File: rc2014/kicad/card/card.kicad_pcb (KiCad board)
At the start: 4 copper layers, 63.5 x 102.6 mm, 27 parts, among them J1 Conn_RC40_Male, J2 DB15_Female_HighDensity, J3 Conn_02x06_Top_Bottom, SW1 SW_DIP_x07, U1 74HCT688, U2 SN74LVC8T245PWR, U3 SN74LVC8T245PWR, U4 VDC-II

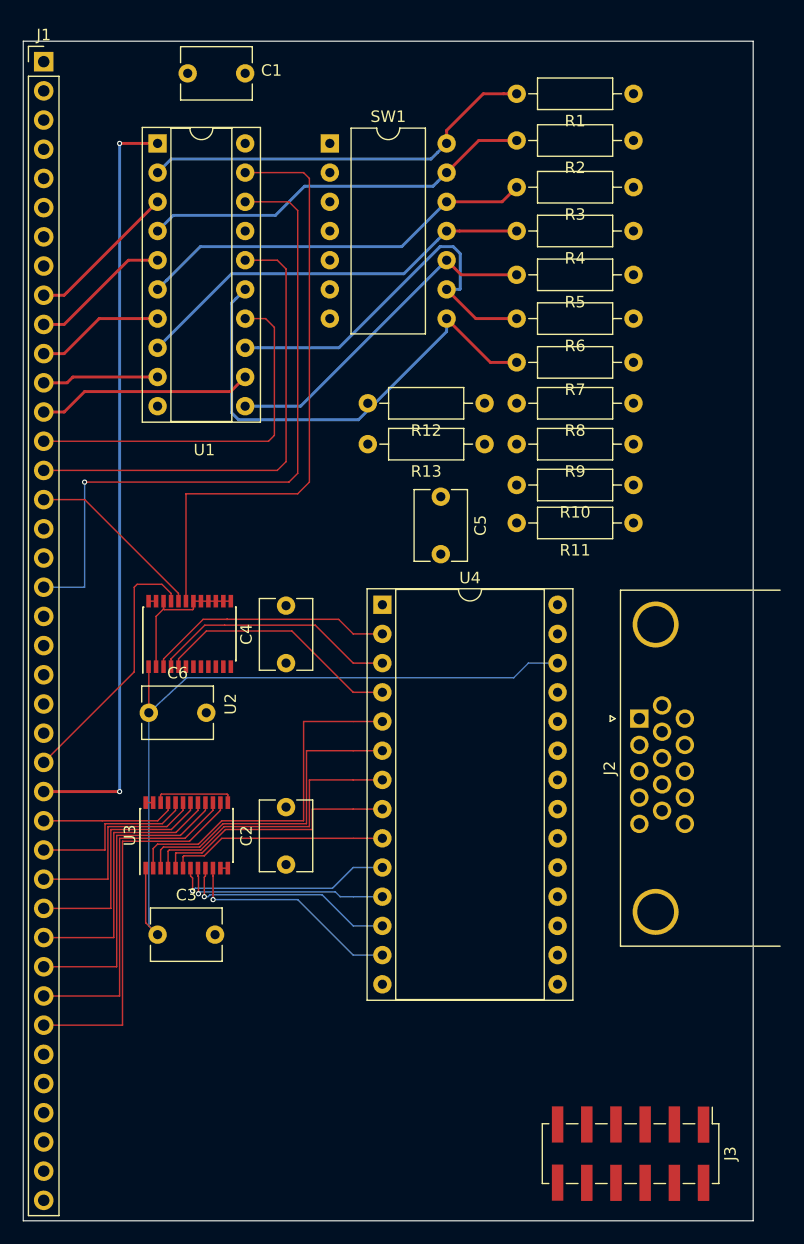
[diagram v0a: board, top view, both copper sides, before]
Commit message: Repin U4
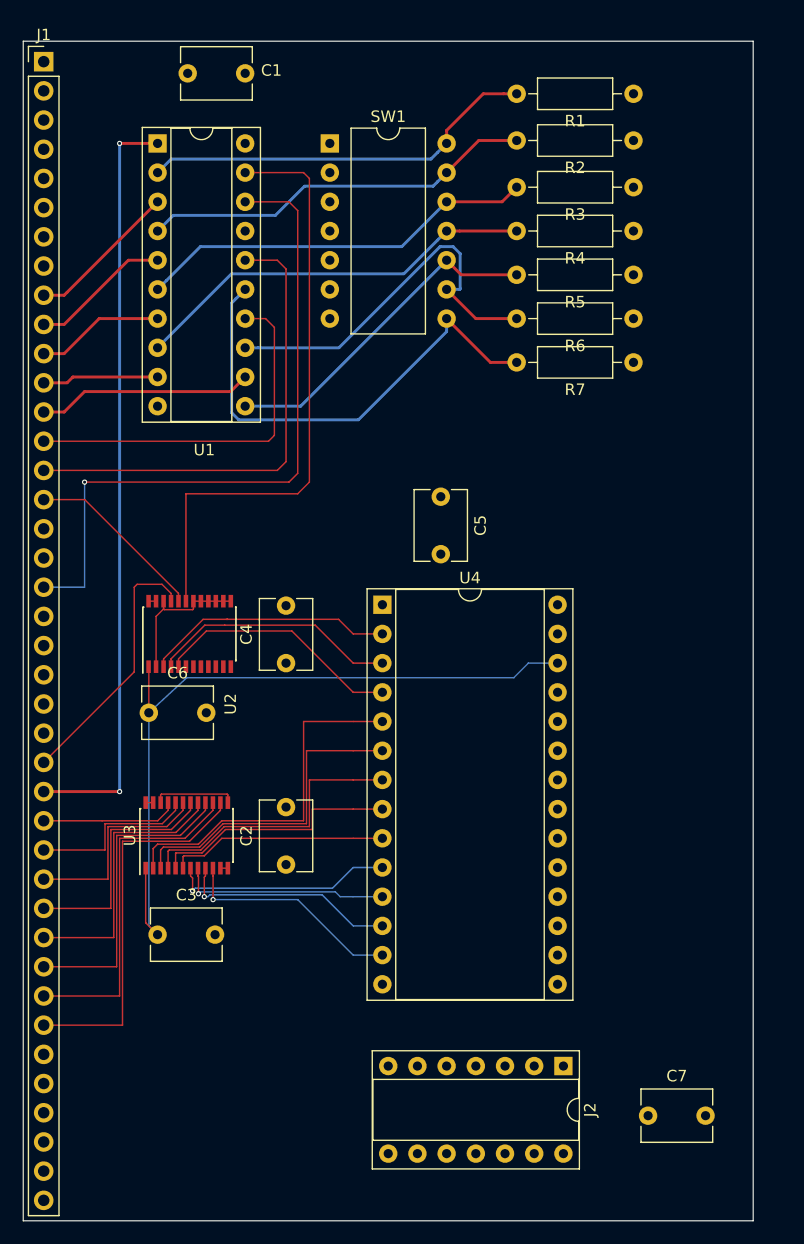
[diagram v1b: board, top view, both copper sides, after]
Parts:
- removed J3: Conn_02x06_Top_Bottom, card:PinHeader_2x06_P2.54mm_Vertical_SMD_top_down
- removed R10, R12, R8: 270, Resistor_THT:R_Axial_DIN0207_L6.3mm_D2.5mm_P10.16mm_Horizontal
- removed R11, R13, R9: 510, Resistor_THT:R_Axial_DIN0207_L6.3mm_D2.5mm_P10.16mm_Horizontal
- added C7: C, Capacitor_THT:C_Disc_D6.0mm_W4.4mm_P5.00mm, F.Cu at (79.8, 118.9)
- J2: value DB15_Female_HighDensity -> VideoMezzanine14; footprint Connector_Dsub:DSUB-15-HD_Female_Horizontal_P2.29x1.98mm_EdgePinOffset8.35mm_Housed_MountingHolesOffset10.89mm -> Package_DIP:DIP-14_W7.62mm_Socket
- U4: value VDC-II -> VDC-II-card
- moved J2 30.9 mm to (72.4, 114.6), turned to 270 degrees
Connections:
- net Net-(J2-Pad14) renamed /R1
- J2 pad 1: Net-(J2-Pad1) -> /R2
- J2 pad 10: GNDD -> /B1
- J2 pad 11: Net-(J2-Pad11) -> +3V3
- J2 pad 12: Net-(J2-Pad12) -> /G0
- J2 pad 13: Net-(J2-Pad13) -> /G2
- J2 pad 2: Net-(J2-Pad2) -> /R0
- J2 pad 3: Net-(J2-Pad3) -> /G1
- J2 pad 4: Net-(J2-Pad4) -> GNDD
- J2 pad 5: GNDD -> /B2
- J2 pad 6: GNDD -> /B0
- J2 pad 7: GNDD -> /HSYNC
- J2 pad 8: GNDD -> /VSYNC
- U4 pad 15: Net-(J2-Pad13) -> /R2
- U4 pad 17: Net-(U4-Pad17) -> /R0
- U4 pad 18: Net-(J3-Pad3) -> /G2
- U4 pad 19: Net-(J3-Pad8) -> /G1
- U4 pad 20: Net-(U4-Pad20) -> /G0
- U4 pad 21: Net-(J3-Pad10) -> /B2
- U4 pad 22: Net-(J3-Pad2) -> /B1
- U4 pad 23: Net-(U4-Pad23) -> /B0
- U4 pad 24: Net-(J3-Pad4) -> /HSYNC
- U4 pad 25: Net-(J3-Pad9) -> /VSYNC
